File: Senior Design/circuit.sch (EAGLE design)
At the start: 16 parts, among them IC2 ATMEGA328P, IC3 ATTINY24A, Q1 16MHz

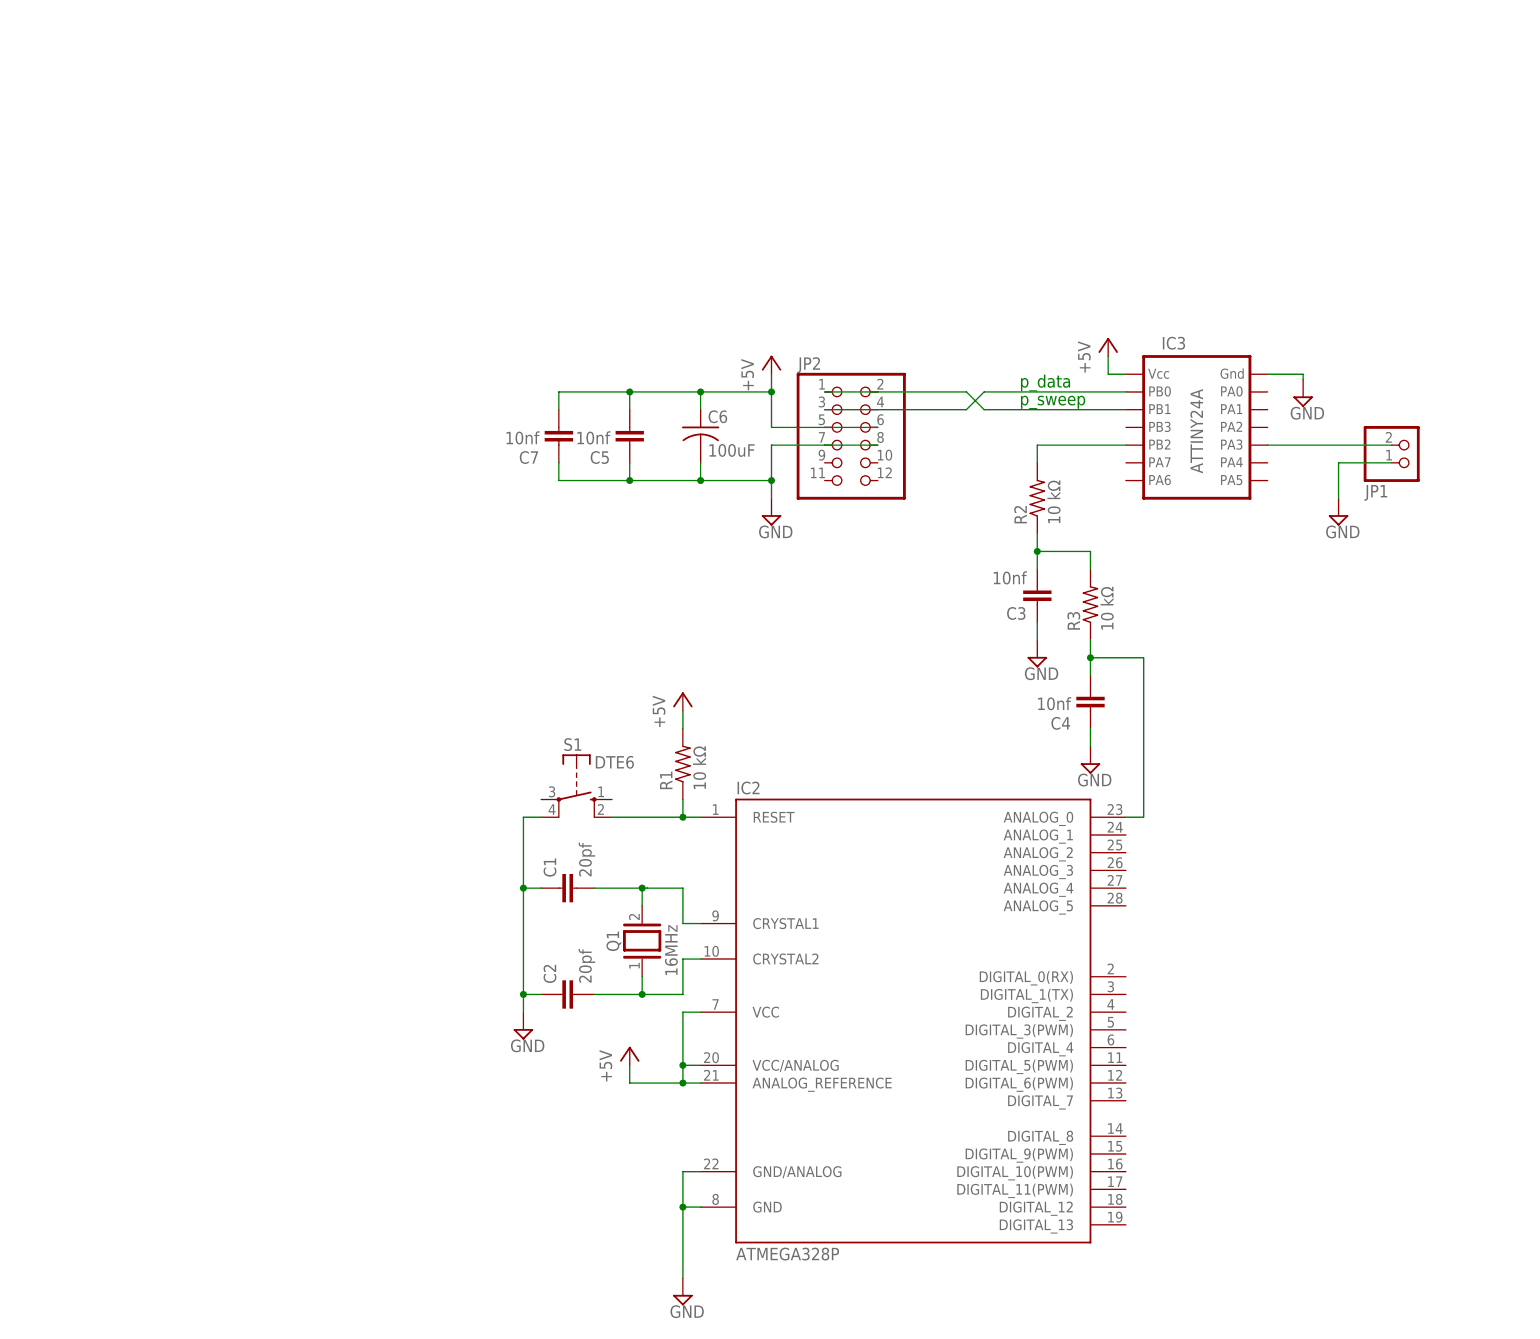
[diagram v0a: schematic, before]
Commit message: worked on the schematic
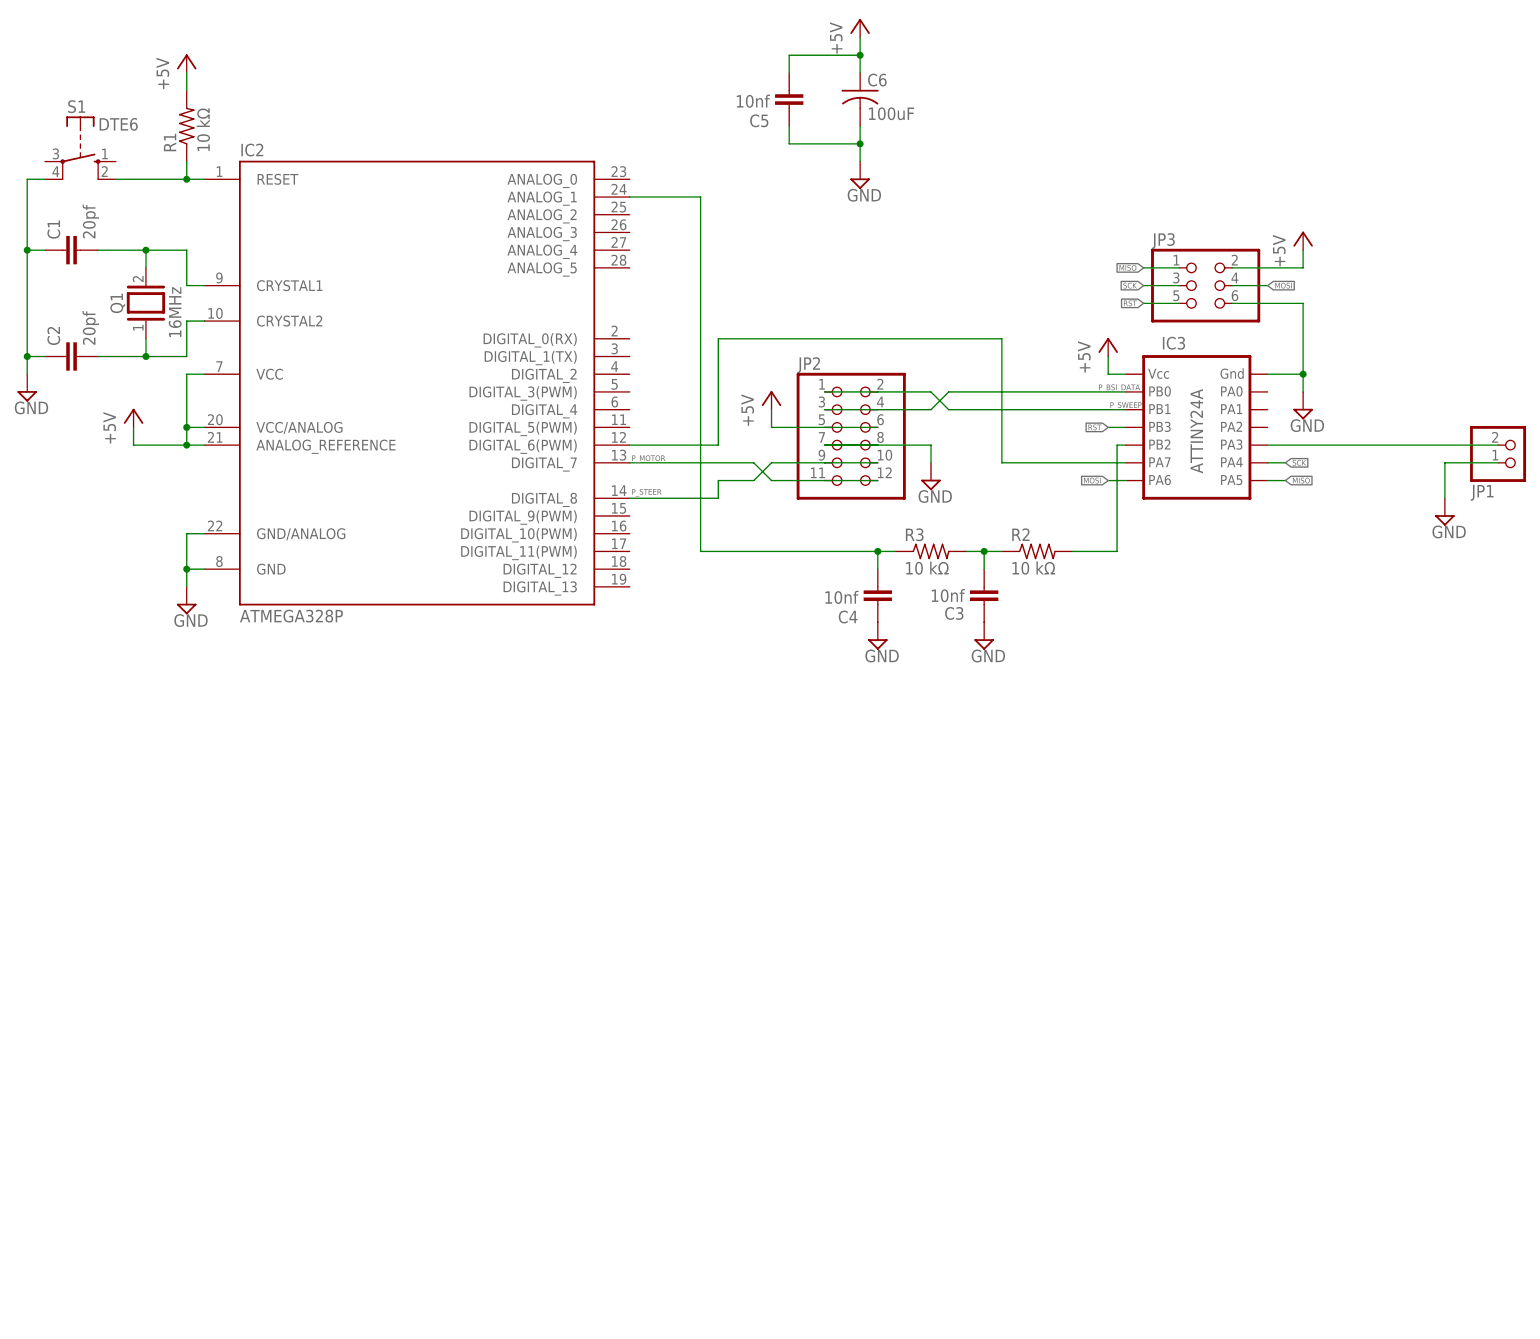
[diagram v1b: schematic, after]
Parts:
- removed C7: 10nf, rcl:C-EU025-024X044
- added JP3: (no value), pinhead:PINHD-2X3
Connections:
- net N$1 renamed P_BSI_DATA
- net N$2 renamed P_SWEEP
- removed net N$9: C4.2, IC2.ANALOG_0, R3.1
- new net DATA-READY: IC2.DIGITAL_6(PWM), IC3.P$6
- new net LINE-POSITION: C4.2, IC2.ANALOG_1, R3.1
- new net MISO: IC3.P$8, JP3.1
- new net MOSI: IC3.P$7, JP3.4
- new net P_MOTOR: IC2.DIGITAL_7, JP2.11, JP2.12
- new net P_STEER: IC2.DIGITAL_8, JP2.10, JP2.9
- new net RST: IC3.P$4, JP3.5
- new net SCK: IC3.P$9, JP3.3
- net +5V: now also JP3.2; no longer C7.2
- net GND: now also JP3.6; no longer C7.1
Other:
- note removed: "p_data"
- note removed: "p_sweep"
- moved on the sheet: C1, C2, C3, C4, C5, C6, IC2, JP1, Q1, R1, R2, R3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
